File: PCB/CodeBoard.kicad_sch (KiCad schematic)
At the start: 161 parts, among them SW1 SW_Push, SW10 SW_Push, SW11 SW_Push, SW12 SW_Push, SW13 SW_Push, SW14 SW_Push, SW15 SW_Push, SW16 SW_Push, SW17 SW_Push, SW18 SW_Push, SW19 SW_Push, SW2 SW_Push, SW20 SW_Push, SW21 SW_Push, SW22 SW_Push, SW23 SW_Push, SW24 SW_Push, SW26 SW_Push, SW27 SW_Push, SW28 SW_Push, SW29 SW_Push, SW3 SW_Push, SW30 SW_Push, SW31 SW_Push, SW32 SW_Push, SW33 SW_Push, SW34 SW_Push, SW35 SW_Push, SW36 SW_Push, SW37 SW_Push, SW38 SW_Push, SW39 SW_Push, SW4 SW_Push, SW40 SW_Push, SW41 SW_Push, SW42 SW_Push, SW43 SW_Push, SW44 SW_Push, SW45 SW_Push, SW46 SW_Push, SW47 SW_Push, SW48 SW_Push, SW49 SW_Push, SW5 SW_Push, SW50 SW_Push, SW51 SW_Push, SW52 SW_Push, SW53 SW_Push, SW54 SW_Push, SW55 SW_Push, SW56 SW_Push, SW57 SW_Push, SW58 SW_Push, SW59 SW_Push, SW6 SW_Push, SW60 SW_Push, SW61 SW_Push, SW62 SW_Push, SW63 SW_Push, SW64 SW_Push, SW65 SW_Push, SW66 SW_Push, SW67 SW_Push, SW68 SW_Push, SW69 SW_Push, SW7 SW_Push, SW70 SW_Push, SW71 SW_Push, SW72 SW_Push, SW73 SW_Push, SW74 SW_Push, SW75 SW_Push, SW76 SW_Push, SW77 SW_Push, SW78 SW_Push, SW79 SW_Push, SW8 SW_Push, SW80 SW_Push, SW81 SW_Push, SW9 SW_Push

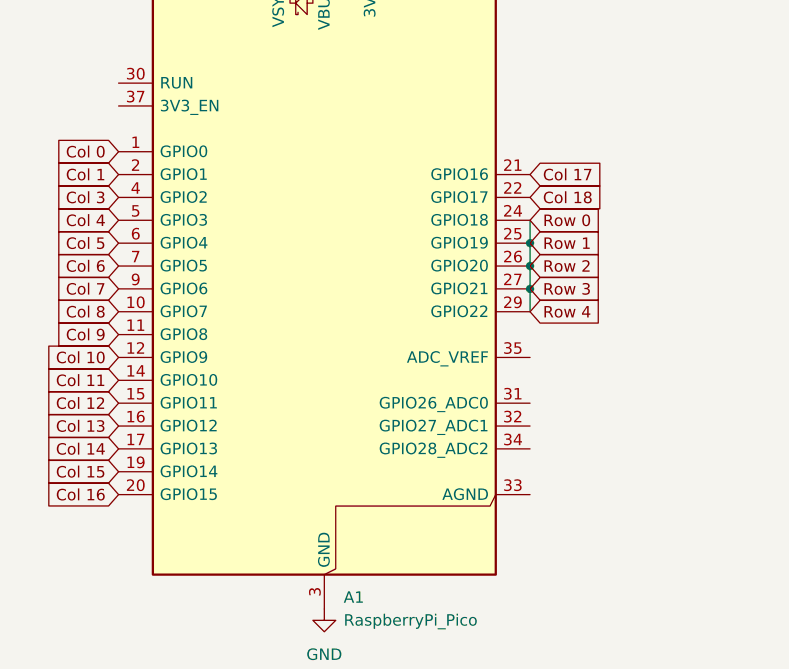
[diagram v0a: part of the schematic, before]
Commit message: Add files via upload
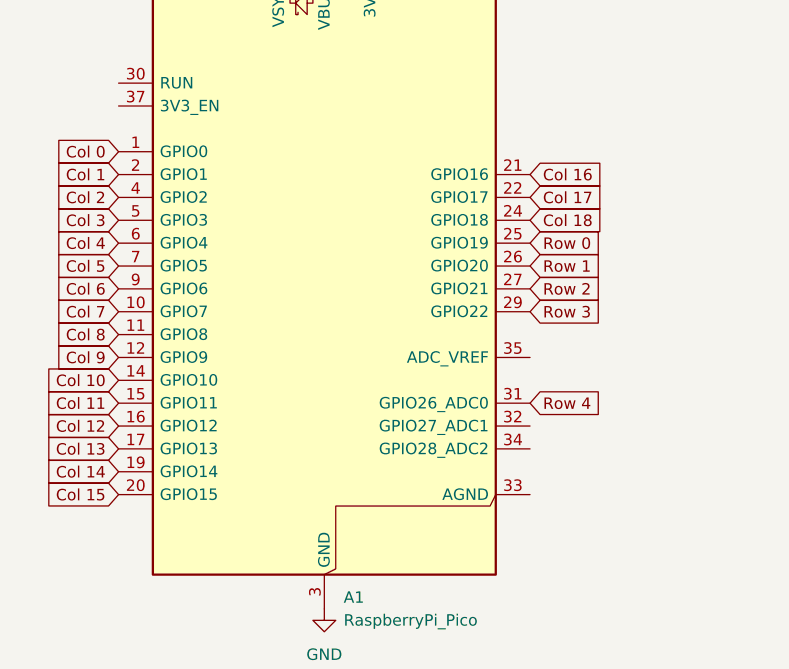
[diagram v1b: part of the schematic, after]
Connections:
- net Col 0: no longer A1.24 (GPIO18), A1.25 (GPIO19), A1.26 (GPIO20), A1.27 (GPIO21), D1.1 (K), D10.1 (K), D11.1 (K), D12.1 (K), D13.1 (K), D14.1 (K), D16.1 (K), D17.1 (K), D18.1 (K), D19.1 (K), D2.1 (K), D20.1 (K), D21.1 (K), D22.1 (K), D23.1 (K), D24.1 (K), D25.1 (K), D26.1 (K), D27.1 (K), D28.1 (K), D29.1 (K), D3.1 (K), D30.1 (K), D31.1 (K), D32.1 (K), D33.1 (K), D34.1 (K), D35.1 (K), D36.1 (K), D37.1 (K), D38.1 (K), D39.1 (K), D4.1 (K), D40.1 (K), D41.1 (K), D42.1 (K), D43.1 (K), D44.1 (K), D45.1 (K), D46.1 (K), D47.1 (K), D48.1 (K), D49.1 (K), D5.1 (K), D50.1 (K), D51.1 (K), D6.1 (K), D69.1 (K), D7.1 (K), D70.1 (K), D71.1 (K), D72.1 (K), D73.1 (K), D74.1 (K), D75.1 (K), D76.1 (K), D77.1 (K), D78.1 (K), D79.1 (K), D8.1 (K), D80.1 (K), D81.1 (K), D9.1 (K), SW30.1, SW35.1
- net Col 18: now reaches A1.31 (GPIO26_ADC0)
- net Col 18: now also A1.24 (GPIO18), D69.1 (K), D70.1 (K), D71.1 (K), D72.1 (K), D73.1 (K), D74.1 (K), D75.1 (K), D76.1 (K), D77.1 (K), D78.1 (K), D79.1 (K), D80.1 (K), D81.1 (K), SW30.1, SW35.1
- new net Row 0: A1.25 (GPIO19), D1.1 (K), D10.1 (K), D11.1 (K), D12.1 (K), D16.1 (K), D17.1 (K), D18.1 (K), D19.1 (K), D2.1 (K), D20.1 (K), D3.1 (K), D4.1 (K), D5.1 (K), D6.1 (K), D7.1 (K), D8.1 (K), D9.1 (K)
- new net Row 1: A1.26 (GPIO20), D13.1 (K), D14.1 (K), D21.1 (K), D22.1 (K), D23.1 (K), D24.1 (K), D25.1 (K), D26.1 (K), D27.1 (K), D28.1 (K), D29.1 (K), D30.1 (K), D31.1 (K), D32.1 (K), D33.1 (K), D34.1 (K), D35.1 (K)
- new net Row 2: A1.27 (GPIO21), D36.1 (K), D37.1 (K), D38.1 (K), D39.1 (K), D40.1 (K), D41.1 (K), D42.1 (K), D43.1 (K), D44.1 (K), D45.1 (K), D46.1 (K), D47.1 (K), D48.1 (K), D49.1 (K), D50.1 (K), D51.1 (K)
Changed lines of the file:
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@@
 	)
 	(junction
-		(at 69.85 158.75)
-		(diameter 0)
-		(color 0 0 0 0)
-	)
-	(junction
 		(at 158.75 118.11)
 		(diameter 0)
@@
 	)
 	(junction
-		(at 69.85 163.83)
-		(diameter 0)
-		(color 0 0 0 0)
-	)
-	(junction
 		(at 120.65 118.11)
 		(diameter 0)
@@
 	)
 	(junction
-		(at 69.85 161.29)
-		(diameter 0)
-		(color 0 0 0 0)
-	)
-	(junction
 		(at 57.15 71.12)
 		(diameter 0)
@@
 	(wire
 		(pts
-			(xy 69.85 156.21) (xy 69.85 158.75)
-		)
-		(stroke
-			(width 0)
-			(type default)
-		)
-	)
-	(wire
-		(pts
 			(xy 44.45 31.75) (xy 44.45 50.8)
 		)
@@
 	(wire
 		(pts
-			(xy 69.85 161.29) (xy 69.85 163.83)
-		)
-		(stroke
-			(width 0)
-			(type default)
-		)
-	)
-	(wire
-		(pts
 			(xy 44.45 91.44) (xy 44.45 99.06)
 		)
@@
 	(wire
 		(pts
-			(xy 69.85 158.75) (xy 69.85 161.29)
-		)
-		(stroke
-			(width 0)
-			(type default)
-		)
-	)
-	(wire
-		(pts
 			(xy 247.65 39.37) (xy 260.35 39.37)
 		)
@@
 	(wire
 		(pts
-			(xy 69.85 163.83) (xy 69.85 166.37)
-		)
-		(stroke
-			(width 0)
-			(type default)
-		)
-	)
-	(wire
-		(pts
 			(xy 110.49 91.44) (xy 110.49 99.06)
 		)
@@
 	(global_label "Col 16"
 		(shape input)
-		(at 24.13 186.69 180)
+		(at 69.85 151.13 0)
 		(fields_autoplaced yes)
 		(effects
@@
 				(size 1.27 1.27)
 			)
-			(justify right)
+			(justify left)
 		)
 		(property "Intersheetrefs" "${INTERSHEET_REFS}"
-			(at 14.674 186.69 0)
+			(at 79.306 151.13 0)
 			(effects
 				(font
 					(size 1.27 1.27)
 				)
-				(justify right)
+				(justify left)
 				(hide yes)
 			)
@@
 	(global_label "Row 3"
 		(shape input)
-		(at 69.85 163.83 0)
+		(at 69.85 166.37 0)
 		(fields_autoplaced yes)
 		(effects
@@
 		)
 		(property "Intersheetrefs" "${INTERSHEET_REFS}"
-			(at 78.7618 163.83 0)
+			(at 78.7618 166.37 0)
 			(effects
 				(font
@@
 	(global_label "Col 8"
 		(shape input)
-		(at 24.13 166.37 180)
+		(at 24.13 168.91 180)
 		(fields_autoplaced yes)
 		(effects
@@
 		)
 		(property "Intersheetrefs" "${INTERSHEET_REFS}"
-			(at 15.8835 166.37 0)
+			(at 15.8835 168.91 0)
 			(effects
 				(font
@@
 	(global_label "Col 18"
 		(shape input)
-		(at 69.85 153.67 0)
+		(at 69.85 156.21 0)
 		(fields_autoplaced yes)
 		(effects
@@
 		)
 		(property "Intersheetrefs" "${INTERSHEET_REFS}"
-			(at 79.306 153.67 0)
+			(at 79.306 156.21 0)
 			(effects
 				(font
@@
 	(global_label "Col 14"
 		(shape input)
-		(at 24.13 181.61 180)
+		(at 24.13 184.15 180)
 		(fields_autoplaced yes)
 		(effects
@@
 		)
 		(property "Intersheetrefs" "${INTERSHEET_REFS}"
-			(at 14.674 181.61 0)
+			(at 14.674 184.15 0)
 			(effects
 				(font
@@
 	(global_label "Row 2"
 		(shape input)
-		(at 69.85 161.29 0)
+		(at 69.85 163.83 0)
 		(fields_autoplaced yes)
 		(effects
@@
 		)
 		(property "Intersheetrefs" "${INTERSHEET_REFS}"
-			(at 78.7618 161.29 0)
+			(at 78.7618 163.83 0)
 			(effects
 				(font
@@
 	(global_label "Col 10"
 		(shape input)
-		(at 24.13 171.45 180)
+		(at 24.13 173.99 180)
 		(fields_autoplaced yes)
 		(effects
@@
 		)
 		(property "Intersheetrefs" "${INTERSHEET_REFS}"
-			(at 14.674 171.45 0)
+			(at 14.674 173.99 0)
 			(effects
 				(font
@@
 	(global_label "Col 4"
 		(shape input)
-		(at 24.13 156.21 180)
+		(at 24.13 158.75 180)
 		(fields_autoplaced yes)
 		(effects
@@
 		)
 		(property "Intersheetrefs" "${INTERSHEET_REFS}"
-			(at 15.8835 156.21 0)
+			(at 15.8835 158.75 0)
 			(effects
 				(font
@@
 	(global_label "Col 3"
 		(shape input)
-		(at 24.13 153.67 180)
+		(at 24.13 156.21 180)
 		(fields_autoplaced yes)
 		(effects
@@
 		)
 		(property "Intersheetrefs" "${INTERSHEET_REFS}"
-			(at 15.8835 153.67 0)
+			(at 15.8835 156.21 0)
 			(effects
 				(font
@@
 	(global_label "Col 6"
 		(shape input)
-		(at 24.13 161.29 180)
+		(at 24.13 163.83 180)
 		(fields_autoplaced yes)
 		(effects
@@
 		)
 		(property "Intersheetrefs" "${INTERSHEET_REFS}"
-			(at 15.8835 161.29 0)
+			(at 15.8835 163.83 0)
+			(effects
+				(font
+					(size 1.27 1.27)
+				)
+				(justify right)
+				(hide yes)
+			)
+		)
+	)
+	(global_label "Col 2"
+		(shape input)
+		(at 24.13 153.67 180)
+		(fields_autoplaced yes)
+		(effects
+			(font
+				(size 1.27 1.27)
+			)
+			(justify right)
+		)
+		(property "Intersheetrefs" "${INTERSHEET_REFS}"
+			(at 15.8835 153.67 0)
 			(effects
 				(font
@@
 	(global_label "Col 5"
 		(shape input)
-		(at 24.13 158.75 180)
+		(at 24.13 161.29 180)
 		(fields_autoplaced yes)
 		(effects
@@
 		)
 		(property "Intersheetrefs" "${INTERSHEET_REFS}"
-			(at 15.8835 158.75 0)
+			(at 15.8835 161.29 0)
 			(effects
 				(font
@@
 	(global_label "Col 7"
 		(shape input)
-		(at 24.13 163.83 180)
+		(at 24.13 166.37 180)
 		(fields_autoplaced yes)
 		(effects
@@
 		)
 		(property "Intersheetrefs" "${INTERSHEET_REFS}"
-			(at 15.8835 163.83 0)
+			(at 15.8835 166.37 0)
 			(effects
 				(font
@@
 	(global_label "Col 11"
 		(shape input)
-		(at 24.13 173.99 180)
+		(at 24.13 176.53 180)
 		(fields_autoplaced yes)
 		(effects
@@
 		)
 		(property "Intersheetrefs" "${INTERSHEET_REFS}"
-			(at 14.674 173.99 0)
+			(at 14.674 176.53 0)
 			(effects
 				(font
@@
 	(global_label "Col 15"
 		(shape input)
-		(at 24.13 184.15 180)
+		(at 24.13 186.69 180)
 		(fields_autoplaced yes)
 		(effects
@@
 		)
 		(property "Intersheetrefs" "${INTERSHEET_REFS}"
-			(at 14.674 184.15 0)
+			(at 14.674 186.69 0)
 			(effects
 				(font
@@
 	(global_label "Row 0"
 		(shape input)
-		(at 69.85 156.21 0)
+		(at 69.85 158.75 0)
 		(fields_autoplaced yes)
 		(effects
@@
 		)
 		(property "Intersheetrefs" "${INTERSHEET_REFS}"
-			(at 78.7618 156.21 0)
+			(at 78.7618 158.75 0)
 			(effects
 				(font
@@
 	(global_label "Row 1"
 		(shape input)
-		(at 69.85 158.75 0)
+		(at 69.85 161.29 0)
 		(fields_autoplaced yes)
 		(effects
@@
 		)
 		(property "Intersheetrefs" "${INTERSHEET_REFS}"
-			(at 78.7618 158.75 0)
+			(at 78.7618 161.29 0)
 			(effects
 				(font
@@
 	(global_label "Col 9"
 		(shape input)
-		(at 24.13 168.91 180)
+		(at 24.13 171.45 180)
 		(fields_autoplaced yes)
 		(effects
@@
 		)
 		(property "Intersheetrefs" "${INTERSHEET_REFS}"
-			(at 15.8835 168.91 0)
+			(at 15.8835 171.45 0)
 			(effects
 				(font
@@
 	(global_label "Col 17"
 		(shape input)
-		(at 69.85 151.13 0)
+		(at 69.85 153.67 0)
 		(fields_autoplaced yes)
 		(effects
@@
 		)
 		(property "Intersheetrefs" "${INTERSHEET_REFS}"
-			(at 79.306 151.13 0)
+			(at 79.306 153.67 0)
 			(effects
 				(font
@@
 	(global_label "Col 13"
 		(shape input)
-		(at 24.13 179.07 180)
+		(at 24.13 181.61 180)
 		(fields_autoplaced yes)
 		(effects
@@
 		)
 		(property "Intersheetrefs" "${INTERSHEET_REFS}"
-			(at 14.674 179.07 0)
+			(at 14.674 181.61 0)
 			(effects
 				(font
@@
 	(global_label "Col 12"
 		(shape input)
-		(at 24.13 176.53 180)
+		(at 24.13 179.07 180)
 		(fields_autoplaced yes)
 		(effects
@@
 		)
 		(property "Intersheetrefs" "${INTERSHEET_REFS}"
-			(at 14.674 176.53 0)
+			(at 14.674 179.07 0)
 			(effects
 				(font
@@
 	(global_label "Row 4"
 		(shape input)
-		(at 69.85 166.37 0)
+		(at 69.85 176.53 0)
 		(fields_autoplaced yes)
 		(effects
@@
 		)
 		(property "Intersheetrefs" "${INTERSHEET_REFS}"
-			(at 78.7618 166.37 0)
+			(at 78.7618 176.53 0)
 			(effects
 				(font
